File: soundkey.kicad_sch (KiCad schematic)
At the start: 28 parts, among them J1 Conn_01x02_Socket, J2 Conn_01x06_Socket, J4 ISD1820, Q1 AO3401A, Q2 AO3401A, U1 ATtiny85-20P, U2 TP4057

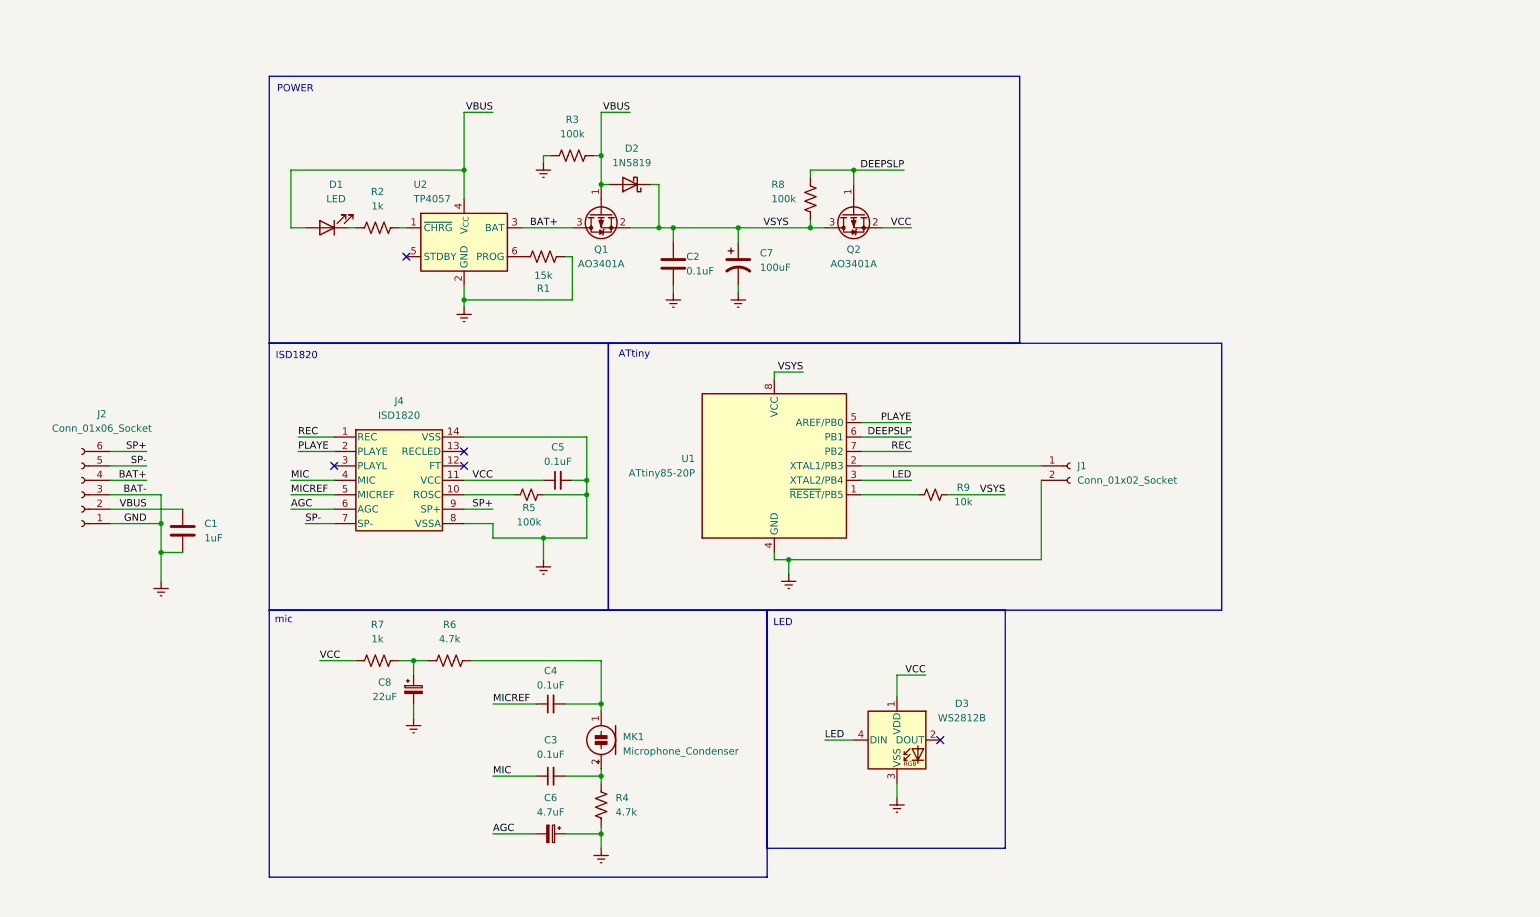
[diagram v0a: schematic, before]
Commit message: 2608292346_thisiswild
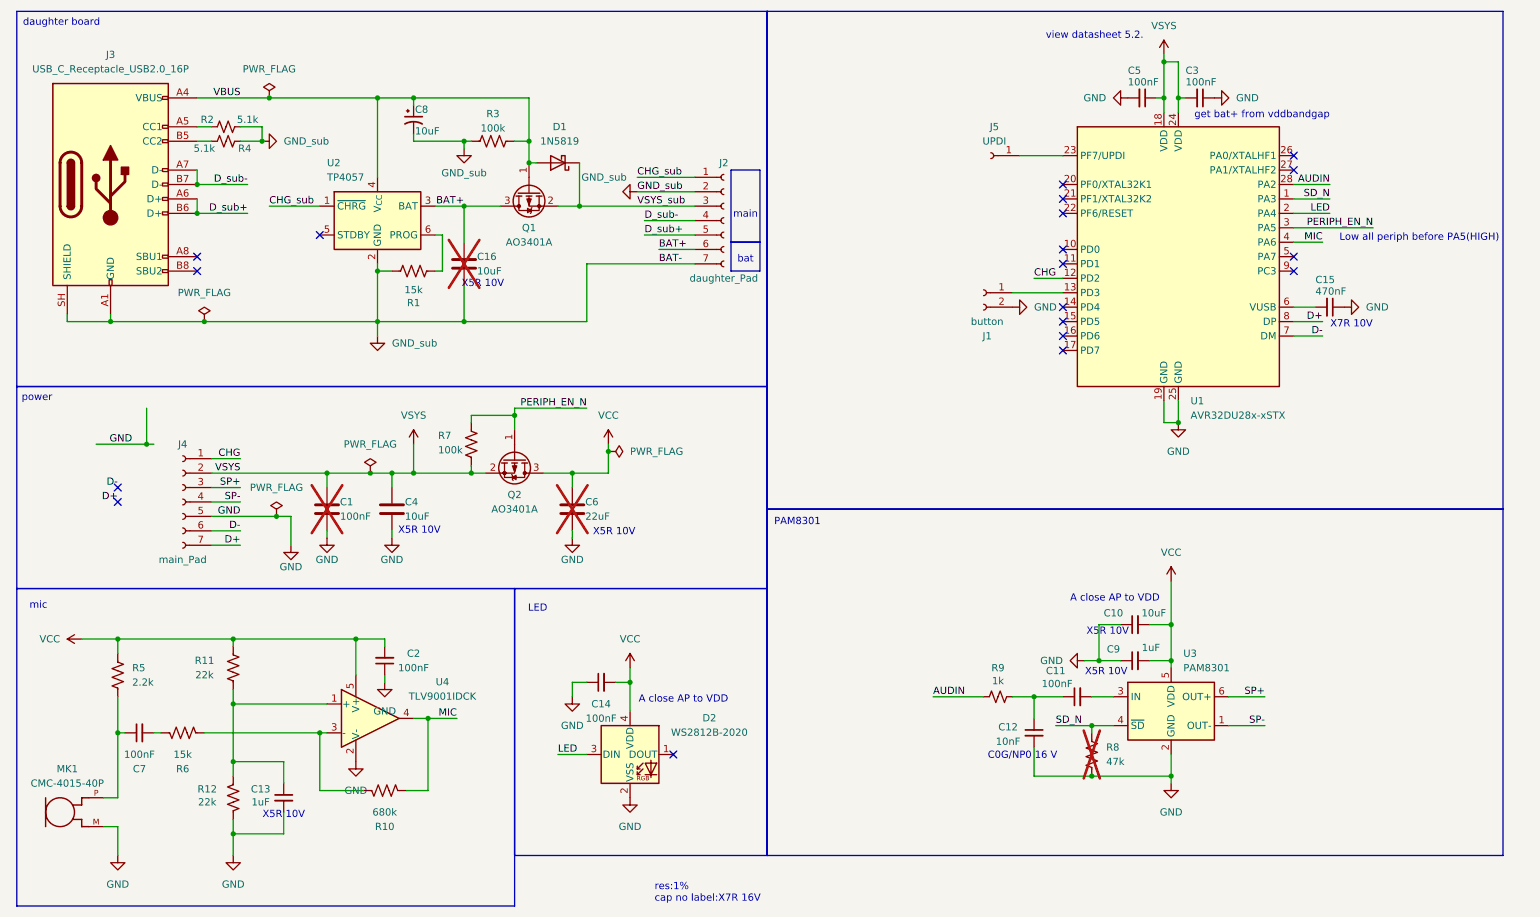
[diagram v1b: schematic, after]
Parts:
- removed C2: 0.1uF, symbol Device:C
- removed C4: 0.1uF, symbol Device:C_Small
- removed C6: 4.7uF, symbol Device:C_Polarized_Small
- removed C7: 100uF, symbol Device:C_Polarized_US
- removed C8: 22uF, symbol Device:C_Polarized_Small
- removed D1: LED, symbol Device:LED
- removed D3: WS2812B, LED_SMD:LED_WS2812B_PLCC4_5.0x5.0mm_P3.2mm, symbol LED:WS2812B
- removed J4: ISD1820, Package_DIP:DIP-14_W7.62mm_Socket, symbol 1_New_Library_0:ISD1820
- removed MK1: Microphone_Condenser, Sensor_Audio:POM-2244P-C3310-2-R, symbol Device:Microphone_Condenser
- removed R2: 1k, symbol Device:R_US
- removed R4: 4.7k, symbol Device:R_US
- removed R5: 100k, symbol Device:R_Small_US
- removed U1: ATtiny85-20P, Package_DIP:DIP-8_W7.62mm, symbol MCU_Microchip_ATtiny:ATtiny85-20P
- added C10: 10uF, Capacitor_SMD:C_0805_2012Metric, symbol Device:C_Small
- added C11, C14, C2, C7: 100nF, Capacitor_SMD:C_0402_1005Metric, symbol Device:C_Small
- added C12: 10nF, Capacitor_SMD:C_0402_1005Metric, symbol Device:C_Small
- added C13, C9: 1uF, Capacitor_SMD:C_0603_1608Metric, symbol Device:C_Small
- added C15: 470nF, Capacitor_SMD:C_0402_1005Metric, symbol Device:C_Small
- added C16, C4: 10uF, Capacitor_SMD:C_0805_2012Metric, symbol Device:C
- added C6: 22uF, Capacitor_SMD:C_1206_3216Metric, symbol Device:C
- added C8: 10uF, Capacitor_THT:C_Radial_D4.0mm_H5.0mm_P1.50mm, symbol Device:C_Polarized_Small_US
- added D2: WS2812B-2020, LED_SMD:LED_WS2812B-2020_PLCC4_2.0x2.0mm, symbol LED:WS2812B-2020
- added J3: USB_C_Receptacle_USB2.0_16P, Connector_USB:USB_C_Receptacle_GCT_USB4105-xx-A_16P_TopMnt_Horizontal, symbol Connector:USB_C_Receptacle_USB2.0_16P
- added J4: main_Pad, 1_Library:Pad_7_1.5x2.0mm_G2.5mm, symbol Connector:Conn_01x07_Socket
- added J5: UPDI, TestPoint:TestPoint_Pad_D1.0mm, symbol Connector:Conn_01x01_Socket
- added MK1: CMC-4015-40P, 1_Library:MIC_CMC-4015-40P, symbol CMC-4015-40P:CMC-4015-40P
- added R10: 680k, Resistor_SMD:R_0603_1608Metric, symbol Device:R_US
- added R11, R12: 22k, Resistor_SMD:R_0402_1005Metric, symbol Device:R_US
- added R2, R4: 5.1k, Resistor_THT:R_Axial_DIN0204_L3.6mm_D1.6mm_P5.08mm_Horizontal, symbol Device:R_Small_US
- added R5: 2.2k, Resistor_SMD:R_0402_1005Metric, symbol Device:R_US
- added U1: AVR32DU28x-xSTX, Package_DFN_QFN:WQFN-28-1EP_4x4mm_P0.4mm_EP2.7x2.7mm_ThermalVias, symbol 1_New_Library_0:AVR64DU28
- added U3: PAM8301, Package_TO_SOT_SMD:SOT-23-6, symbol Amplifier_Audio:PAM8301
- added U4: TLV9001IDCK, Package_TO_SOT_SMD:SOT-353_SC-70-5, symbol Amplifier_Operational:TLV9001IDCK
- C1: value 1uF -> 100nF; footprint (none) -> Capacitor_SMD:C_0402_1005Metric; now not fitted
- C3, C5: value 0.1uF -> 100nF; footprint (none) -> Capacitor_SMD:C_0402_1005Metric
- D1: renamed from D2; footprint Diode_THT:D_DO-41_SOD81_P10.16mm_Horizontal -> Diode_THT:D_DO-41_SOD81_P7.62mm_Horizontal
- J1: value Conn_01x02_Socket -> button
- J2: value Conn_01x06_Socket -> daughter_Pad; footprint (none) -> 1_Library:Pad_7_1.5x2.0mm_G2.5mm; symbol Connector:Conn_01x06_Socket -> Connector:Conn_01x07_Socket
- R1, R3: footprint (none) -> Resistor_THT:R_Axial_DIN0204_L3.6mm_D1.6mm_P5.08mm_Horizontal
- R6: value 4.7k -> 15k; footprint (none) -> Resistor_SMD:R_0402_1005Metric
- R7: value 1k -> 100k; footprint (none) -> Resistor_SMD:R_0402_1005Metric
- R8: value 100k -> 47k; footprint (none) -> Resistor_SMD:R_0402_1005Metric; now not fitted
- R9: value 10k -> 1k; footprint (none) -> Resistor_SMD:R_0402_1005Metric
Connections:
- net BAT+: now also J2.6 (Pin_6), C16.1; no longer J2.4 (Pin_4)
- net LED: now also D2.3 (DIN), U1.2 (PA4)
- net MIC: now also R10.1, U1.4 (PA6), U4.4; no longer C3.1
- net SP+: now also J4.3 (Pin_3), U3.6 (OUT+); no longer J2.6 (Pin_6)
- net SP-: now also J4.4 (Pin_4), U3.1 (OUT-); no longer J2.5 (Pin_5)
- net VBUS: now also C8.1, J3.A4 (VBUS), J3.A9 (VBUS), J3.B4 (VBUS), J3.B9 (VBUS); no longer C1.1, J2.2 (Pin_2)
- net VCC: now also Q2.3 (D), C10.2, C14.2, C2.2, C6.1, C9.2, D2.4 (VDD), R11.1, R5.1, U3.5 (VDD), U4.5 (V+); no longer C5.1, Q2.2 (S), R7.2
- net VSYS: now also C1.1, C3.2, C5.1, Q2.2 (S), R7.1, C4.1, J4.2 (Pin_2), U1.18 (VDD), U1.24 (VDD); no longer D1.1 (K), Q1.2 (S), Q2.3 (D), R8.1, R9.2
- net at R9.1: now also C11.1, C12.1
- net at J1.1 (Pin_1): now also U1.13 (PD3)
- net at R6.1: now also R10.2, U4.3 (-)
- net at R6.2: now also C7.2; no longer R7.1
- net CHG_sub: now reaches U2.1 (~{CHRG})
- net CHG_sub: now also J2.1 (Pin_1)
- net at U2.6 (PROG): now also R1.2; no longer R1.1
- net DEEPSLP renamed PERIPH_EN_N
- net PERIPH_EN_N: now also R7.2, U1.3 (PA5); no longer R8.2
- removed net Earth: C1.2, C5.2, J1.2 (Pin_2), J2.1 (Pin_1), J2.3 (Pin_3), R1.2, R3.1, U2.2 (GND)
- new net: C13.1, R11.2, R12.1, U4.1 (+)
- new net: C7.1, MK1.P, R5.2
- new net: J3.B5 (CC2), R4.1
- new net: J3.A5 (CC1), R2.2
- new net: J5.1 (Pin_1), U1.23 (PF7/UPDI)
- new net: C15.2, U1.6 (VUSB)
- new net: C11.2, U3.3 (IN)
- new net AUDIN: R9.2, U1.28 (PA2)
- new net CHG: J4.1 (Pin_1), U1.12 (PD2)
- new net D+: J4.7 (Pin_7), U1.8 (DP)
- new net D-: J4.6 (Pin_6), U1.7 (DM)
- new net D_sub+: J2.5 (Pin_5), J3.A6 (D+), J3.B6 (D+)
- new net D_sub-: J2.4 (Pin_4), J3.A7 (D-), J3.B7 (D-)
- new net GND: C1.2, C10.1, C12.2, C13.2, C14.1, C15.1, C2.1, C3.1, C4.2, C5.2, C6.2, C9.1, D2.2 (VSS), J1.2 (Pin_2), J4.5 (Pin_5), MK1.M, R12.2, R8.1, U1.19 (GND), U1.25 (GND), U1.29 (GND_EP), U3.2 (GND), U4.2 (V-)
- new net GND_sub: C16.2, C8.2, J2.2 (Pin_2), J2.7 (Pin_7), J3.A1 (GND), J3.A12 (GND), J3.B1 (GND), J3.B12 (GND), J3.SH (SHIELD), R1.1, R2.1, R3.1, R4.2, U2.2 (GND)
- new net SD_N: R8.2, U1.1 (PA3), U3.4 (~{SD})
- new net VSYS_sub: D1.1 (K), J2.3 (Pin_3), Q1.2 (S)
- no-connect marks 5 -> 19
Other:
- note added: "A close AP to VDD"
- note added: "C0G/NP0 16 V"
- note added: "Low all periph before PA5(HIGH)"
- note added: "PAM8301"
- note added: "X5R 10V"
- note added: "X7R 10V"
- note added: "bat"
- note added: "daughter board"
- note added: "get bat+ from vddbandgap"
- note added: "main"
- note added: "power"
- note added: "res:1% cap no label:X7R 16V"
- note added: "view datasheet 5.2."
- note removed: "ATtiny"
- note removed: "ISD1820"
- note removed: "POWER"
- moved on the sheet: D1, Q1, R3, U2

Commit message: 2608300232_half wire
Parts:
- C11, C7: footprint Capacitor_SMD:C_0402_1005Metric -> Capacitor_SMD:C_0603_1608Metric
- R10: footprint Resistor_SMD:R_0603_1608Metric -> Resistor_SMD:R_0402_1005Metric
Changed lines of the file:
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@@
 			)
 		)
-		(property "Footprint" "Capacitor_SMD:C_0402_1005Metric"
+		(property "Footprint" "Capacitor_SMD:C_0603_1608Metric"
 			(at 40.64 142.24 0)
 			(hide yes)
@@
 			)
 		)
-		(property "Footprint" "Resistor_SMD:R_0603_1608Metric"
+		(property "Footprint" "Resistor_SMD:R_0402_1005Metric"
 			(at 83.566 151.384 90)
 			(hide yes)
@@
 			)
 		)
-		(property "Footprint" "Capacitor_SMD:C_0402_1005Metric"
+		(property "Footprint" "Capacitor_SMD:C_0603_1608Metric"
 			(at 205.74 135.89 0)
 			(hide yes)
